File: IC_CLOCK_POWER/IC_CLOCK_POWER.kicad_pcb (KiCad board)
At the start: 2 copper layers, 90.1 x 58.4 mm, 24 parts, among them J1 Conn_01x02_Pin, J2 Conn_01x04_Pin, U1 LM7805_TO220_HEAT_SINK, U2 LM317T

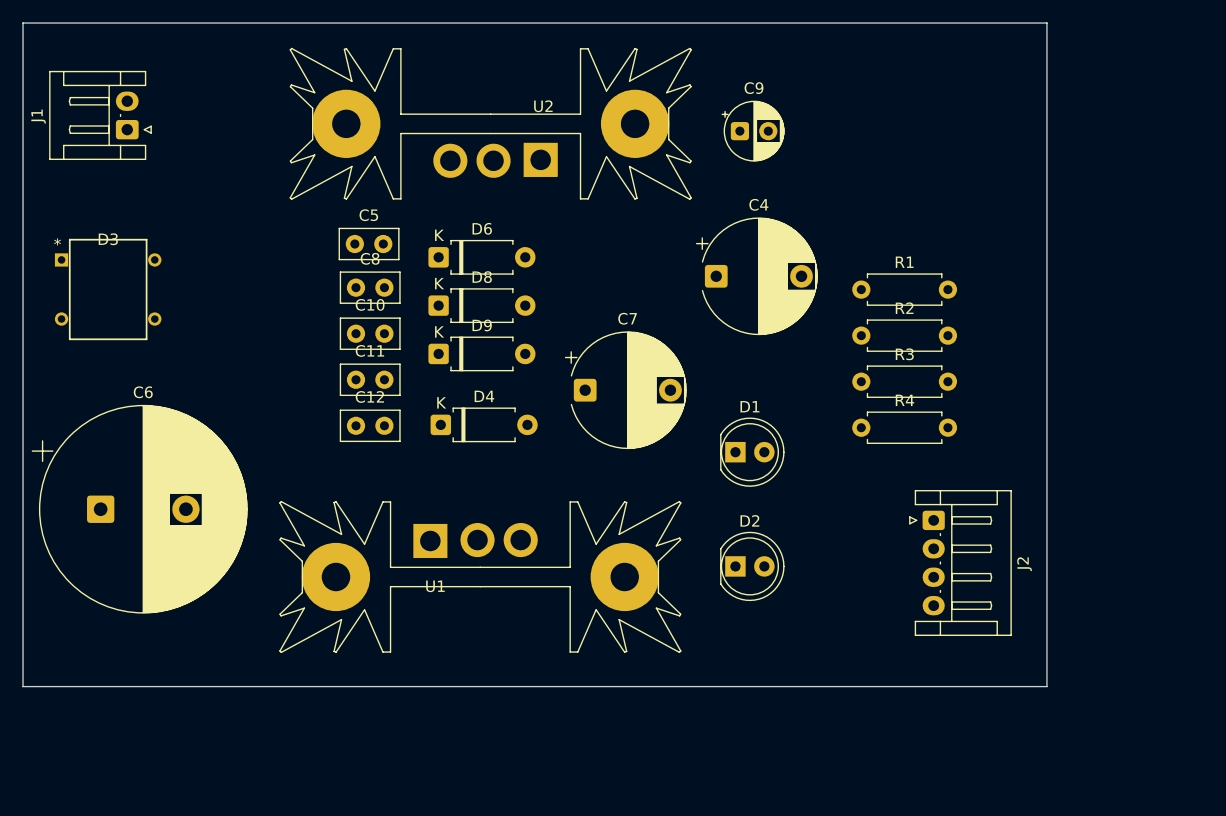
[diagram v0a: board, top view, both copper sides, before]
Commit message: Update to files ...
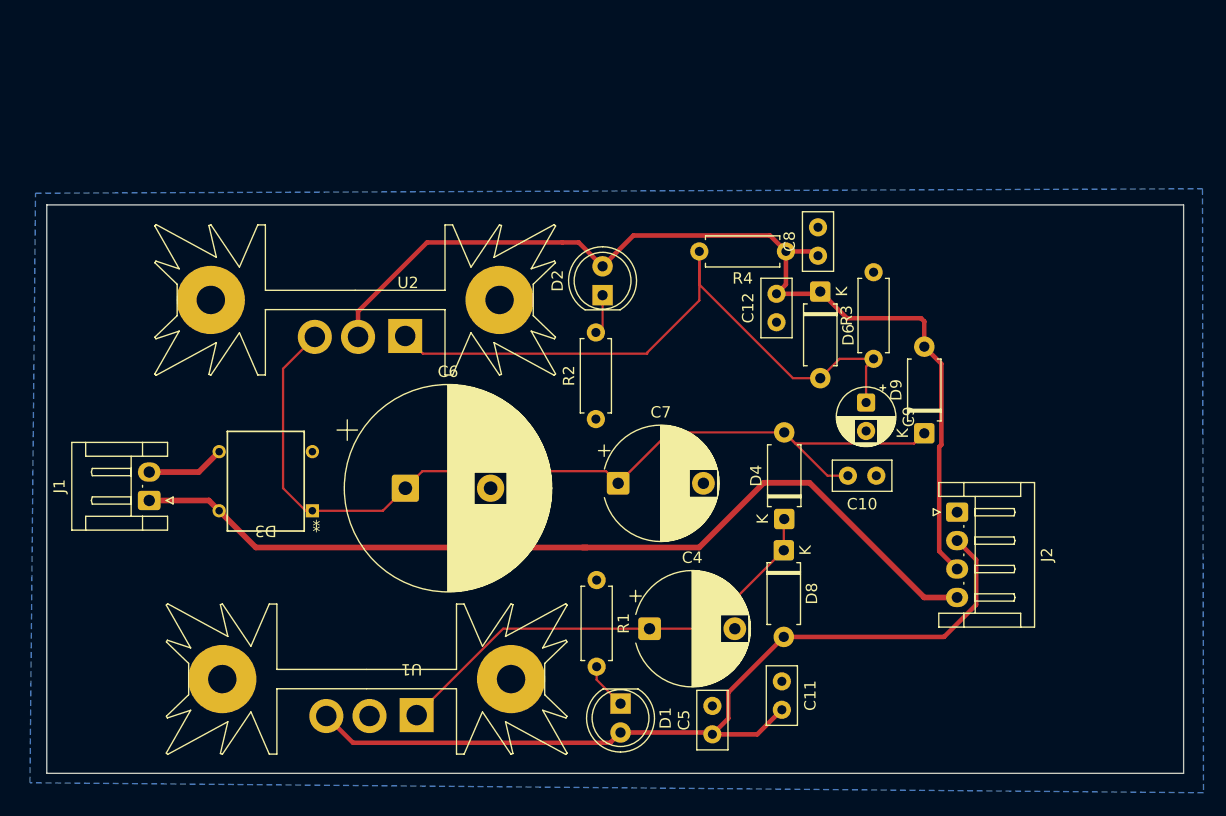
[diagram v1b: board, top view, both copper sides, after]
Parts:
- moved C5 53.4 mm to (158.6, 146.6), turned to 90 degrees
- moved C10 47.4 mm to (173.0, 123.8), turned to 180 degrees
- moved C11 45.9 mm to (164.7, 141.9), turned to -90 degrees
- moved D9 43.3 mm to (177.2, 120.1), turned to 90 degrees
- moved C8 40.7 mm to (167.8, 104.5), turned to 90 degrees
- moved C12 38.1 mm to (164.2, 110.3), turned to 90 degrees
- moved D8 37.2 mm to (164.8, 130.4), turned to -90 degrees
- moved R1 34.6 mm to (148.4, 133.0), turned to -90 degrees
- moved D6 33.7 mm to (168.0, 107.6), turned to -90 degrees
- moved J1 32.7 mm to (109.0, 126.0)
- moved C4 31.6 mm to (153.0, 137.3)
- moved D4 31.3 mm to (164.9, 127.6), turned to 90 degrees
- moved C6 26.9 mm to (131.5, 124.9)
- moved D2 26.6 mm to (148.9, 107.9), turned to 90 degrees
- moved C9 26.3 mm to (172.1, 117.4), turned to -90 degrees
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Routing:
- net +10V: track 0.00 -> 89.3 mm
- net Net-(D3-+): track 0.00 -> 84.4 mm
- net 12VAC: track 0.00 -> 79.8 mm
- net +5V: track 0.00 -> 78.0 mm
- net Net-(D6-A): track 0.00 -> 59.3 mm
- net Net-(D4-K): track 0.00 -> 41.1 mm
- net AC-GND: track 0.00 -> 6.90 mm
- net Net-(D1-K): track 0.00 -> 4.12 mm
- net Net-(D2-K): track 0.00 -> 4.01 mm
- added copper zone on B.Cu, net GND
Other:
- board size 90.1 x 58.4 mm -> 100 x 50 mm
